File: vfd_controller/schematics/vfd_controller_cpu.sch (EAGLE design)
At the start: 35 parts, among them IC1 Atmega1284P, IC2 Attiny861A, J1 , J2 , X1 20MHz, X10 JST-XH-04-PIN-LONG-PAD, X11 JST-XH-04-PIN-LONG-PAD, X12 JST-XH-04-PIN-LONG-PAD, X13 JST-XH-07-PIN-LONG-PAD, X2 JST-XH-02-PIN-LONG-PAD, X3 JST-XH-02-PIN-LONG-PAD, X4 JST-XH-04-PIN-LONG-PAD, X5 JST-XH-10-PIN-LONG-PAD, X6 JST-XH-02-PIN-LONG-PAD, X7 JST-XH-04-PIN-LONG-PAD, X8 JST-XH-04-PIN-LONG-PAD, X9 JST-XH-04-PIN-LONG-PAD

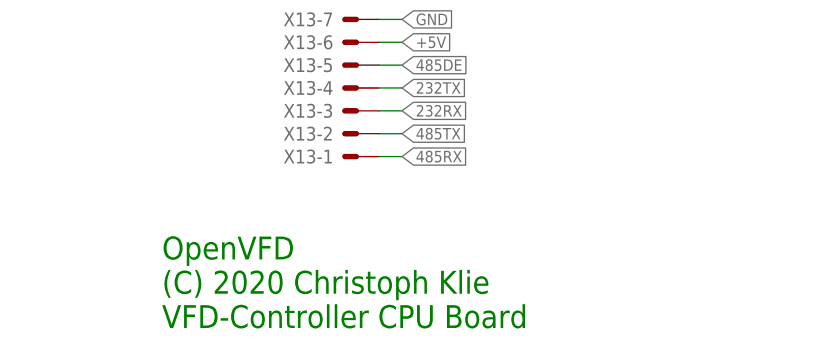
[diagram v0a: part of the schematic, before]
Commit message: Minor changes to Schematics Changed IGBT-Driver signal-side connector to plugs Updated Schematic Information Field
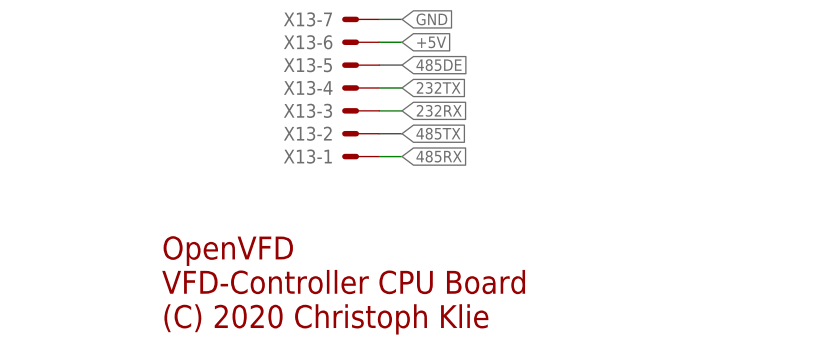
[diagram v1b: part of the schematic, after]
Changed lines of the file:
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@@
 <setting verticaltext="up"/>
 </settings>
-<grid distance="0.1" unitdist="inch" unit="inch" style="lines" multiple="1" display="no" altdistance="0.01" altunitdist="inch" altunit="inch"/>
+<grid distance="0.05" unitdist="inch" unit="inch" style="lines" multiple="1" display="no" altdistance="0.01" altunitdist="inch" altunit="inch"/>
 <layers>
 <layer number="1" name="Top" color="4" fill="1" visible="no" active="no"/>
@@
 <text x="60.96" y="172.72" size="1.27" layer="91">OVER 485</text>
 <text x="96.52" y="88.9" size="1.27" layer="91" rot="R180">DEBUG</text>
-<text x="163.83" y="31.75" size="2.54" layer="91">OpenVFD</text>
-<text x="163.83" y="27.94" size="2.54" layer="91">(C) 2020 Christoph Klie</text>
-<text x="163.83" y="24.13" size="2.54" layer="91">VFD-Controller CPU Board</text>
+<text x="163.83" y="31.75" size="2.54" layer="94">OpenVFD</text>
+<text x="163.83" y="24.13" size="2.54" layer="94">(C) 2020 Christoph Klie</text>
+<text x="163.83" y="27.94" size="2.54" layer="94">VFD-Controller CPU Board</text>
 </plain>
 <instances>
